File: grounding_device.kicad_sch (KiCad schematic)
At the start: 144 parts, among them IC1 NE555P, IC2 NE555P, IC3 NE555P, IC4 NE555P, Q1 2N2222, Q10 2N2222, Q11 2N2222, Q12 2N2222, Q2 2N2222, Q3 2N2222, Q4 2N2222, Q5 2N2222, Q6 2N2222, Q7 2N2222, Q8 2N2222, Q9 2N2222

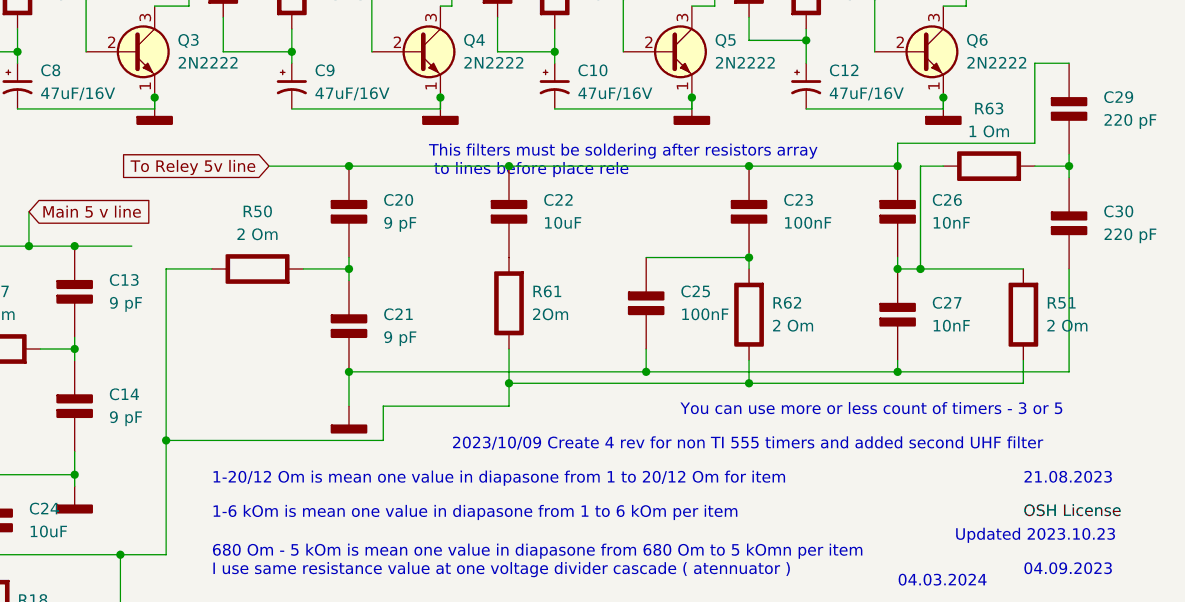
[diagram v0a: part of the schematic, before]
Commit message: Upgrade
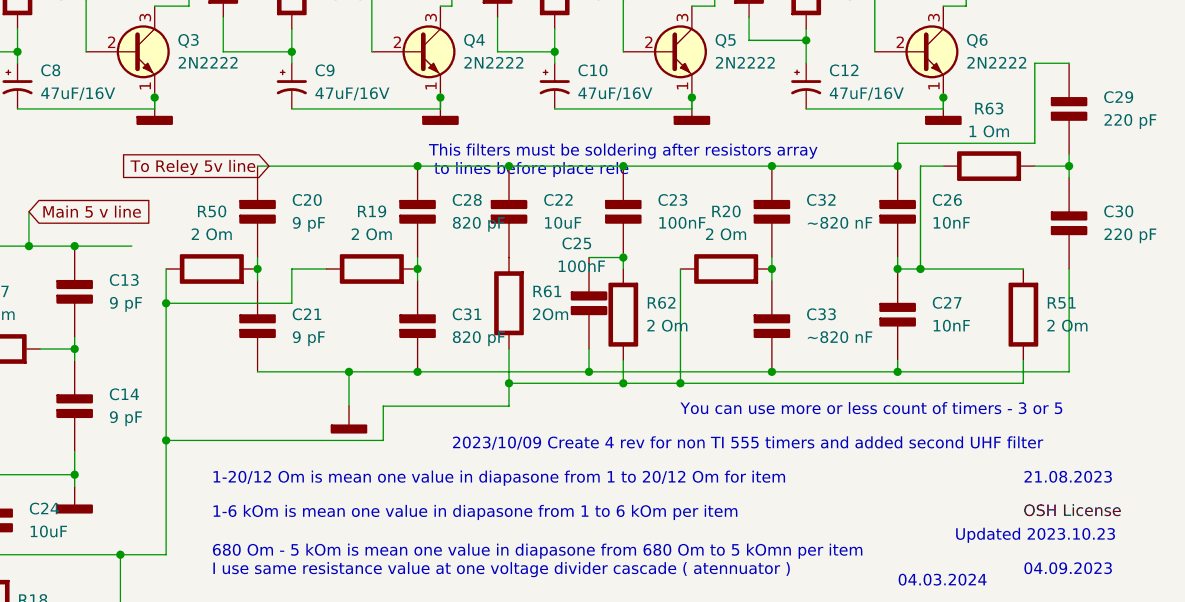
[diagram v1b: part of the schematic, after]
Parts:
- added C28, C31: 820 pF, symbol PCM_Elektuur:C
- added C32, C33: ~820 nF, symbol PCM_Elektuur:C
- added R19, R20: 2 Om, symbol PCM_Elektuur:R
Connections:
- net 0: now also C31.2 (-), C33.2 (-)
- net Filters/Ground: now also R19.1 (+), R20.1 (+)
- net To Reley 5v line : now also C28.1 (+), C32.1 (+)
- new net: C32.2 (-), C33.1 (+), R20.2 (-)
- new net: C28.2 (-), C31.1 (+), R19.2 (-)
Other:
- moved on the sheet: C20, C21, C23, C25, R50, R62

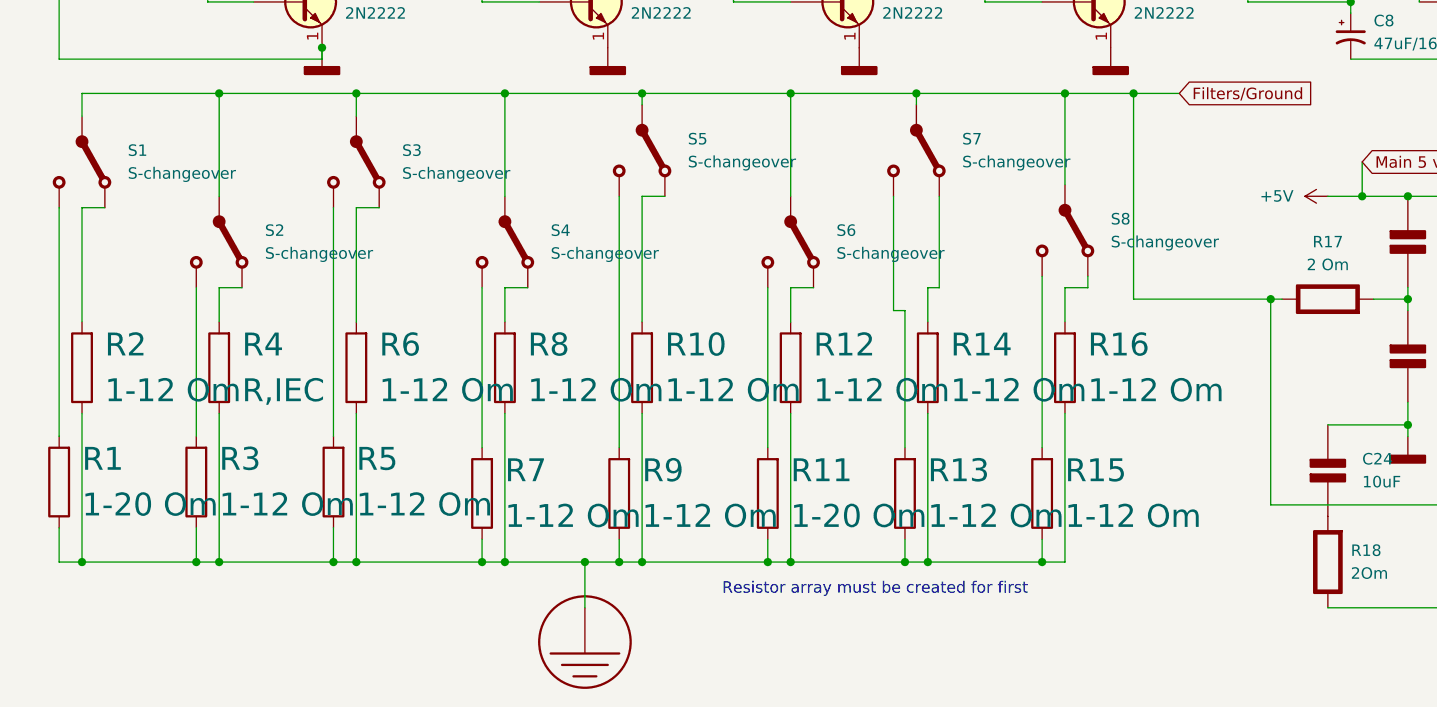
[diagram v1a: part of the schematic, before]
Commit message: Upgarade
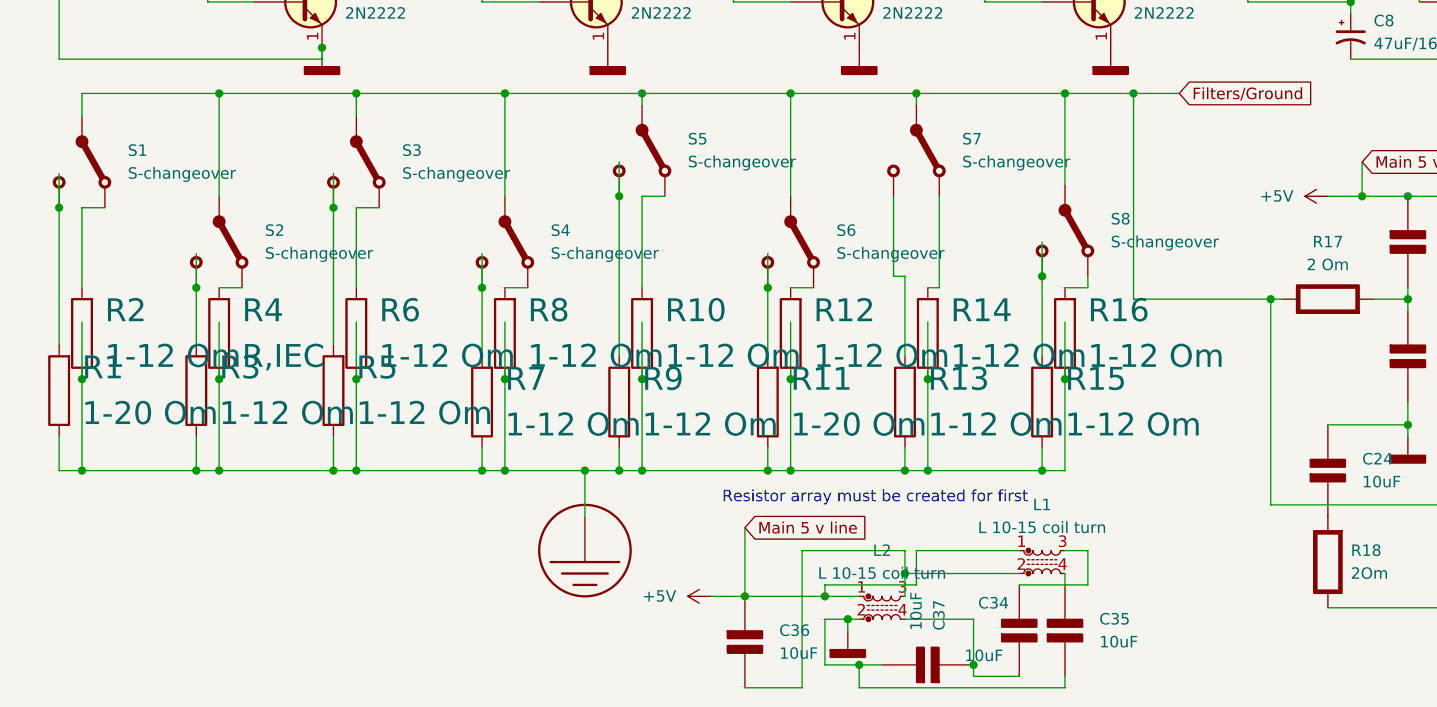
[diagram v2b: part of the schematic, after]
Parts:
- added C34, C35, C36, C37: 10uF, symbol PCM_Elektuur:C
- added L1, L2: L 10-15 coil turn, symbol Device:L_Ferrite_Coupled_Small_1324
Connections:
- net +5V: now also C36.1 (+), L1.1, L2.1
- net 0: now also C35.2 (-), C37.2 (-), L2.2
- new net: C35.1 (+), L1.4
- new net: C36.2 (-), L1.2, L2.3
- new net: C34.1 (+), L1.3
- new net: C34.2 (-), C37.1 (+), L2.4
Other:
- moved on the sheet: R1, R10, R11, R12, R13, R14, R15, R16, R2, R3, R4, R5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
